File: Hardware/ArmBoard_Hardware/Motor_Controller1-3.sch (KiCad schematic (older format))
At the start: 27 parts, among them Q31 BUK7M6R3-40EX, Q32 BUK7M6R3-40EX, Q33 BUK7M6R3-40EX, U3 VNH5019A_E, U4 VNH5019A_E, U5 VNH5019A_E

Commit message: need to change the mosfet and the other footrpints under it
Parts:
- R40, R41, R42, R43, R44, R45, R46, R47, R48, R49, R50, R51, R52, R53, R54, R55, R56, R57, R58, R59, R60: footprint (none) -> Resistor_SMD:R_0603_1608Metric_Pad0.98x0.95mm_HandSolder
- U3, U4, U5: footprint (none) -> MRDT_ICs:MultiPowerSO_30
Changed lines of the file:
@@
 F 0 "U5" H 3550 4137 60  0000 C CNN
 F 1 "VNH5019A_E" H 3550 4031 60  0000 C CNN
-F 2 "" H 2950 3750 60  0001 C CNN
+F 2 "MRDT_ICs:MultiPowerSO_30" H 2950 3750 60  0001 C CNN
 F 3 "" H 2950 3750 60  0001 C CNN
 	1    2950 2450
@@
 F 0 "R60" H 2700 1350 50  0000 R CNN
 F 1 "3.3k" H 2700 1450 50  0000 R CNN
-F 2 "" H 2500 1400 50  0001 C CNN
+F 2 "Resistor_SMD:R_0603_1608Metric_Pad0.98x0.95mm_HandSolder" H 2500 1400 50  0001 C CNN
 F 3 "~" H 2500 1400 50  0001 C CNN
 	1    2500 1400
@@
 F 0 "R57" V 2450 1550 50  0000 C CNN
 F 1 "1k" V 2350 1550 50  0000 C CNN
-F 2 "" H 2350 1550 50  0001 C CNN
+F 2 "Resistor_SMD:R_0603_1608Metric_Pad0.98x0.95mm_HandSolder" H 2350 1550 50  0001 C CNN
 F 3 "~" H 2350 1550 50  0001 C CNN
 	1    2350 1550
@@
 F 0 "R52" H 2309 2646 50  0000 L CNN
 F 1 "3.3k" H 2309 2555 50  0000 L CNN
-F 2 "" H 2250 2600 50  0001 C CNN
+F 2 "Resistor_SMD:R_0603_1608Metric_Pad0.98x0.95mm_HandSolder" H 2250 2600 50  0001 C CNN
 F 3 "~" H 2250 2600 50  0001 C CNN
 	1    2250 2600
@@
 F 0 "R48" V 2200 2750 50  0000 C CNN
 F 1 "1k" V 2100 2750 50  0000 C CNN
-F 2 "" H 2100 2750 50  0001 C CNN
+F 2 "Resistor_SMD:R_0603_1608Metric_Pad0.98x0.95mm_HandSolder" H 2100 2750 50  0001 C CNN
 F 3 "~" H 2100 2750 50  0001 C CNN
 	1    2100 2750
@@
 F 0 "U3" H 3450 8787 60  0000 C CNN
 F 1 "VNH5019A_E" H 3450 8681 60  0000 C CNN
-F 2 "" H 2850 8400 60  0001 C CNN
+F 2 "MRDT_ICs:MultiPowerSO_30" H 2850 8400 60  0001 C CNN
 F 3 "" H 2850 8400 60  0001 C CNN
 	1    2850 7100
@@
 F 0 "R58" H 2600 6000 50  0000 R CNN
 F 1 "3.3k" H 2600 6100 50  0000 R CNN
-F 2 "" H 2400 6050 50  0001 C CNN
+F 2 "Resistor_SMD:R_0603_1608Metric_Pad0.98x0.95mm_HandSolder" H 2400 6050 50  0001 C CNN
 F 3 "~" H 2400 6050 50  0001 C CNN
 	1    2400 6050
@@
 F 0 "R54" V 2350 6200 50  0000 C CNN
 F 1 "1k" V 2250 6200 50  0000 C CNN
-F 2 "" H 2250 6200 50  0001 C CNN
+F 2 "Resistor_SMD:R_0603_1608Metric_Pad0.98x0.95mm_HandSolder" H 2250 6200 50  0001 C CNN
 F 3 "~" H 2250 6200 50  0001 C CNN
 	1    2250 6200
@@
 F 0 "R49" H 2209 7296 50  0000 L CNN
 F 1 "3.3k" H 2209 7205 50  0000 L CNN
-F 2 "" H 2150 7250 50  0001 C CNN
+F 2 "Resistor_SMD:R_0603_1608Metric_Pad0.98x0.95mm_HandSolder" H 2150 7250 50  0001 C CNN
 F 3 "~" H 2150 7250 50  0001 C CNN
 	1    2150 7250
@@
 F 0 "R44" V 2100 7400 50  0000 C CNN
 F 1 "1k" V 2000 7400 50  0000 C CNN
-F 2 "" H 2000 7400 50  0001 C CNN
+F 2 "Resistor_SMD:R_0603_1608Metric_Pad0.98x0.95mm_HandSolder" H 2000 7400 50  0001 C CNN
 F 3 "~" H 2000 7400 50  0001 C CNN
 	1    2000 7400
@@
 F 0 "U4" H 3500 6437 60  0000 C CNN
 F 1 "VNH5019A_E" H 3500 6331 60  0000 C CNN
-F 2 "" H 2900 6050 60  0001 C CNN
+F 2 "MRDT_ICs:MultiPowerSO_30" H 2900 6050 60  0001 C CNN
 F 3 "" H 2900 6050 60  0001 C CNN
 	1    2900 4750
@@
 F 0 "R59" H 2650 3650 50  0000 R CNN
 F 1 "3.3k" H 2650 3750 50  0000 R CNN
-F 2 "" H 2450 3700 50  0001 C CNN
+F 2 "Resistor_SMD:R_0603_1608Metric_Pad0.98x0.95mm_HandSolder" H 2450 3700 50  0001 C CNN
 F 3 "~" H 2450 3700 50  0001 C CNN
 	1    2450 3700
@@
 F 0 "R56" V 2400 3850 50  0000 C CNN
 F 1 "1k" V 2300 3850 50  0000 C CNN
-F 2 "" H 2300 3850 50  0001 C CNN
+F 2 "Resistor_SMD:R_0603_1608Metric_Pad0.98x0.95mm_HandSolder" H 2300 3850 50  0001 C CNN
 F 3 "~" H 2300 3850 50  0001 C CNN
 	1    2300 3850
@@
 F 0 "R50" H 2259 4946 50  0000 L CNN
 F 1 "3.3k" H 2259 4855 50  0000 L CNN
-F 2 "" H 2200 4900 50  0001 C CNN
+F 2 "Resistor_SMD:R_0603_1608Metric_Pad0.98x0.95mm_HandSolder" H 2200 4900 50  0001 C CNN
 F 3 "~" H 2200 4900 50  0001 C CNN
 	1    2200 4900
@@
 F 0 "R47" V 2150 5050 50  0000 C CNN
 F 1 "1k" V 2050 5050 50  0000 C CNN
-F 2 "" H 2050 5050 50  0001 C CNN
+F 2 "Resistor_SMD:R_0603_1608Metric_Pad0.98x0.95mm_HandSolder" H 2050 5050 50  0001 C CNN
 F 3 "~" H 2050 5050 50  0001 C CNN
 	1    2050 5050
@@
 F 0 "R43" V 1900 4400 50  0000 C CNN
 F 1 "1k" V 2000 4400 50  0000 C CNN
-F 2 "" H 2000 4400 50  0001 C CNN
+F 2 "Resistor_SMD:R_0603_1608Metric_Pad0.98x0.95mm_HandSolder" H 2000 4400 50  0001 C CNN
 F 3 "~" H 2000 4400 50  0001 C CNN
 	1    2000 4400
@@
 F 0 "R42" V 1900 4150 50  0000 C CNN
 F 1 "1k" V 2000 4150 50  0000 C CNN
-F 2 "" H 2000 4150 50  0001 C CNN
+F 2 "Resistor_SMD:R_0603_1608Metric_Pad0.98x0.95mm_HandSolder" H 2000 4150 50  0001 C CNN
 F 3 "~" H 2000 4150 50  0001 C CNN
 	1    2000 4150
@@
 F 0 "R53" V 2150 4300 50  0000 C CNN
 F 1 "1k" V 2250 4300 50  0000 C CNN
-F 2 "" H 2250 4300 50  0001 C CNN
+F 2 "Resistor_SMD:R_0603_1608Metric_Pad0.98x0.95mm_HandSolder" H 2250 4300 50  0001 C CNN
 F 3 "~" H 2250 4300 50  0001 C CNN
 	1    2250 4300
@@
 F 0 "R41" V 1850 6750 50  0000 C CNN
 F 1 "1k" V 1950 6750 50  0000 C CNN
-F 2 "" H 1950 6750 50  0001 C CNN
+F 2 "Resistor_SMD:R_0603_1608Metric_Pad0.98x0.95mm_HandSolder" H 1950 6750 50  0001 C CNN
 F 3 "~" H 1950 6750 50  0001 C CNN
 	1    1950 6750
@@
 F 0 "R40" V 1850 6500 50  0000 C CNN
 F 1 "1k" V 1950 6500 50  0000 C CNN
-F 2 "" H 1950 6500 50  0001 C CNN
+F 2 "Resistor_SMD:R_0603_1608Metric_Pad0.98x0.95mm_HandSolder" H 1950 6500 50  0001 C CNN
 F 3 "~" H 1950 6500 50  0001 C CNN
 	1    1950 6500
@@
 F 0 "R51" V 2100 6650 50  0000 C CNN
 F 1 "1k" V 2200 6650 50  0000 C CNN
-F 2 "" H 2200 6650 50  0001 C CNN
+F 2 "Resistor_SMD:R_0603_1608Metric_Pad0.98x0.95mm_HandSolder" H 2200 6650 50  0001 C CNN
 F 3 "~" H 2200 6650 50  0001 C CNN
 	1    2200 6650
@@
 F 0 "R46" V 1950 2100 50  0000 C CNN
 F 1 "1k" V 2050 2100 50  0000 C CNN
-F 2 "" H 2050 2100 50  0001 C CNN
+F 2 "Resistor_SMD:R_0603_1608Metric_Pad0.98x0.95mm_HandSolder" H 2050 2100 50  0001 C CNN
 F 3 "~" H 2050 2100 50  0001 C CNN
 	1    2050 2100
@@
 F 0 "R45" V 1950 1850 50  0000 C CNN
 F 1 "1k" V 2050 1850 50  0000 C CNN
-F 2 "" H 2050 1850 50  0001 C CNN
+F 2 "Resistor_SMD:R_0603_1608Metric_Pad0.98x0.95mm_HandSolder" H 2050 1850 50  0001 C CNN
 F 3 "~" H 2050 1850 50  0001 C CNN
 	1    2050 1850
@@
 F 0 "R55" V 2200 2000 50  0000 C CNN
 F 1 "1k" V 2300 2000 50  0000 C CNN
-F 2 "" H 2300 2000 50  0001 C CNN
+F 2 "Resistor_SMD:R_0603_1608Metric_Pad0.98x0.95mm_HandSolder" H 2300 2000 50  0001 C CNN
 F 3 "~" H 2300 2000 50  0001 C CNN
 	1    2300 2000

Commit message: late night with the boy
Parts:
- removed Q31, Q32, Q33: BUK7M6R3-40EX, Package_TO_SOT_SMD:LFPAK33, symbol Transistor_FET:BUK7M6R3-40EX
- removed R40, R41, R42, R43, R44, R45, R46, R47, R48, R51, R53, R54, R55, R56, R57: 1k, Resistor_SMD:R_0603_1608Metric_Pad0.98x0.95mm_HandSolder, symbol Device:R_Small
- removed R49, R50, R52, R58, R59, R60: 3.3k, Resistor_SMD:R_0603_1608Metric_Pad0.98x0.95mm_HandSolder, symbol Device:R_Small
- removed U3, U4, U5: VNH5019A_E, MRDT_ICs:MultiPowerSO_30, symbol ArmBoard_Hardware-rescue:VNH5019A_E-MRDT_ICs
- added C5, C6, C7: C_Small, Capacitor_SMD:C_0603_1608Metric_Pad1.08x0.95mm_HandSolder, symbol Device:C_Small
- added R26, R27, R32: 20k, Resistor_SMD:R_0603_1608Metric_Pad0.98x0.95mm_HandSolder, symbol Device:R
- added R28, R29, R30, R31, R33, R34: 1k, Resistor_SMD:R_0603_1608Metric_Pad0.98x0.95mm_HandSolder, symbol Device:R_Small
- added U4, U5, U8: LTC6900, Package_TO_SOT_SMD:SOT-23-5_HandSoldering, symbol MRDT_Devices:LTC6900
- added U6, U7, U9: TB67H400AFNG,EL, MRDT_ICs:TB67H400AFNG,EL, symbol MRDT_ICs:TB67H400AFNG,EL
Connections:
- net labels added: +5V
- net labels removed: +3.3V, ENa_1, ENa_2, ENa_3, ENb_1, ENb_2, ENb_3
- wire segments 228 -> 165
- no-connect marks 0 -> 12

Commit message: Fixed Oscillators
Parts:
- C5, C6, C7: value C_Small -> .1uF
- U4, U5, U8: symbol MRDT_Devices:LTC6900 -> ArmBoard_Hardware-rescue:LTC6900-MRDT_Devices
- U6, U7, U9: symbol MRDT_ICs:TB67H400AFNG,EL -> ArmBoard_Hardware-rescue:TB67H400AFNG,EL-MRDT_ICs
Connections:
- net +5V: now also R26.1, R27.2, R32.2
- net GND: now also C5.2, C6.2, C7.2
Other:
- moved on the sheet: C5, C6, C7, R27
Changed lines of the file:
@@
 	1035 775  1035 740
 Wire Wire Line
-	825  775  1035 775
+	705  775  880  775
 Wire Wire Line
 	1210 775  1210 925
@@
 $EndComp
 Wire Wire Line
-	825  1125 830  1125
-Wire Wire Line
-	825  975  825  1125
+	880  1125 890  1125
 $Comp
 L Device:C_Small C6
 U 1 1 61CA53E2
-P 825 875
-F 0 "C6" H 917 921 50  0000 L CNN
-F 1 "C_Small" H 917 830 50  0000 L CNN
-F 2 "Capacitor_SMD:C_0603_1608Metric_Pad1.08x0.95mm_HandSolder" H 825 875 50  0001 C CNN
-F 3 "~" H 825 875 50  0001 C CNN
-	1    825  875
-	1    0    0    -1
-$EndComp
-Wire Wire Line
-	1130 1125 1210 1125
-$Comp
-L Device:R R27
-U 1 1 61AA62F2
-P 980 1125
-F 0 "R27" V 1187 1125 50  0000 C CNN
-F 1 "20k" V 1096 1125 50  0000 C CNN
-F 2 "Resistor_SMD:R_0603_1608Metric_Pad0.98x0.95mm_HandSolder" V 910 1125 50  0001 C CNN
-F 3 "~" H 980 1125 50  0001 C CNN
-	1    980  1125
-	0    1    1    0
-$EndComp
-Wire Wire Line
-	705  1025 1210 1025
+P 705 875
+F 0 "C6" H 510 935 50  0000 L CNN
+F 1 ".1uF" H 470 875 50  0000 L CNN
+F 2 "Capacitor_SMD:C_0603_1608Metric_Pad1.08x0.95mm_HandSolder" H 705 875 50  0001 C CNN
+F 3 "~" H 705 875 50  0001 C CNN
+	1    705  875
+	1    0    0    -1
+$EndComp
+Wire Wire Line
+	1190 1125 1210 1125
 NoConn ~ 1210 1225
 $Comp
@@
 	1850 1025 2390 1025
 $Comp
-L MRDT_Devices:LTC6900 U5
+L ArmBoard_Hardware-rescue:LTC6900-MRDT_Devices U5
 U 1 1 6198744B
 P 1460 985
+AR Path="/6198744B" Ref="U5"  Part="1"
+AR Path="/63845F20/6198744B" Ref="U5"  Part="1"
 F 0 "U5" H 1530 1270 50  0000 C CNN
 F 1 "LTC6900" H 1530 1179 50  0000 C CNN
@@
 IN_A_2
 $Comp
-L MRDT_ICs:TB67H400AFNG,EL U9
+L ArmBoard_Hardware-rescue:TB67H400AFNG,EL-MRDT_ICs U9
 U 1 1 620C9E6A
 P 8605 2385
@@
 	7580 1435 7805 1435
 $Comp
-L MRDT_Devices:LTC6900 U8
+L ArmBoard_Hardware-rescue:LTC6900-MRDT_Devices U8
 U 1 1 620C9E19
 P 6875 995
+AR Path="/620C9E19" Ref="U8"  Part="1"
+AR Path="/63845F20/620C9E19" Ref="U8"  Part="1"
 F 0 "U8" H 6945 1280 50  0000 C CNN
 F 1 "LTC6900" H 6945 1189 50  0000 C CNN
@@
 L Device:C_Small C7
 U 1 1 620C9DFD
-P 6240 885
-F 0 "C7" H 6332 931 50  0000 L CNN
-F 1 "C_Small" H 6332 840 50  0000 L CNN
-F 2 "Capacitor_SMD:C_0603_1608Metric_Pad1.08x0.95mm_HandSolder" H 6240 885 50  0001 C CNN
-F 3 "~" H 6240 885 50  0001 C CNN
-	1    6240 885
-	1    0    0    -1
-$EndComp
-Wire Wire Line
-	6240 985  6240 1135
+P 6120 895
+F 0 "C7" H 6212 941 50  0000 L CNN
+F 1 ".1uF" H 6212 850 50  0000 L CNN
+F 2 "Capacitor_SMD:C_0603_1608Metric_Pad1.08x0.95mm_HandSolder" H 6120 895 50  0001 C CNN
+F 3 "~" H 6120 895 50  0001 C CNN
+	1    6120 895
+	1    0    0    -1
+$EndComp
 Wire Wire Line
 	6240 1135 6245 1135
@@
 	6625 785  6625 935
 Wire Wire Line
-	6240 785  6450 785
-Wire Wire Line
 	6450 785  6450 750
 Connection ~ 6450 785
@@
 Wire Wire Line
 	815  4725 820  4725
-Wire Wire Line
-	815  4575 815  4725
 $Comp
 L Device:C_Small C5
 U 1 1 621A2B7A
-P 815 4475
-F 0 "C5" H 907 4521 50  0000 L CNN
-F 1 "C_Small" H 907 4430 50  0000 L CNN
-F 2 "Capacitor_SMD:C_0603_1608Metric_Pad1.08x0.95mm_HandSolder" H 815 4475 50  0001 C CNN
-F 3 "~" H 815 4475 50  0001 C CNN
-	1    815  4475
+P 695 4480
+F 0 "C5" H 787 4526 50  0000 L CNN
+F 1 ".1uF" H 787 4435 50  0000 L CNN
+F 2 "Capacitor_SMD:C_0603_1608Metric_Pad1.08x0.95mm_HandSolder" H 695 4480 50  0001 C CNN
+F 3 "~" H 695 4480 50  0001 C CNN
+	1    695  4480
 	1    0    0    -1
 $EndComp
@@
 	1840 4625 2380 4625
 $Comp
-L MRDT_Devices:LTC6900 U4
+L ArmBoard_Hardware-rescue:LTC6900-MRDT_Devices U4
 U 1 1 621A2B96
 P 1450 4585
+AR Path="/621A2B96" Ref="U4"  Part="1"
+AR Path="/63845F20/621A2B96" Ref="U4"  Part="1"
 F 0 "U4" H 1520 4870 50  0000 C CNN
 F 1 "LTC6900" H 1520 4779 50  0000 C CNN
@@
 	3180 7525 3180 7400
 $Comp
-L MRDT_ICs:TB67H400AFNG,EL U6
+L ArmBoard_Hardware-rescue:TB67H400AFNG,EL-MRDT_ICs U6
 U 1 1 621A2BE7
 P 3180 5975
@@
 OUTa_3
 $Comp
-L MRDT_ICs:TB67H400AFNG,EL U7
+L ArmBoard_Hardware-rescue:TB67H400AFNG,EL-MRDT_ICs U7
 U 1 1 61982ADA
 P 3190 2375
@@
 	1    0    0    -1
 $EndComp
+$Comp
+L Device:R R27
+U 1 1 61AA62F2
+P 1040 1125
+F 0 "R27" V 1247 1125 50  0000 C CNN
+F 1 "20k" V 1156 1125 50  0000 C CNN
+F 2 "Resistor_SMD:R_0603_1608Metric_Pad0.98x0.95mm_HandSolder" V 970 1125 50  0001 C CNN
+F 3 "~" H 1040 1125 50  0001 C CNN
+	1    1040 1125
+	0    1    1    0
+$EndComp
+Wire Wire Line
+	705  1025 1210 1025
+Wire Wire Line
+	705  975  705  1025
+Connection ~ 705  1025
+Wire Wire Line
+	880  1125 880  775
+Connection ~ 880  775
+Wire Wire Line
+	880  775  1035 775
+Wire Wire Line
+	695  4580 695  4625
+Connection ~ 695  4625
+Wire Wire Line
+	815  4375 815  4725
+Wire Wire Line
+	815  4375 695  4375
+Wire Wire Line
+	695  4375 695  4380
+Connection ~ 815  4375
+Wire Wire Line
+	6120 795  6120 785
+Wire Wire Line
+	6120 785  6240 785
+Connection ~ 6240 785
+Wire Wire Line
+	6240 785  6450 785
+Wire Wire Line
+	6240 785  6240 1135
+Wire Wire Line
+	6120 995  6120 1035
+Connection ~ 6120 1035
 $EndSCHEMATC

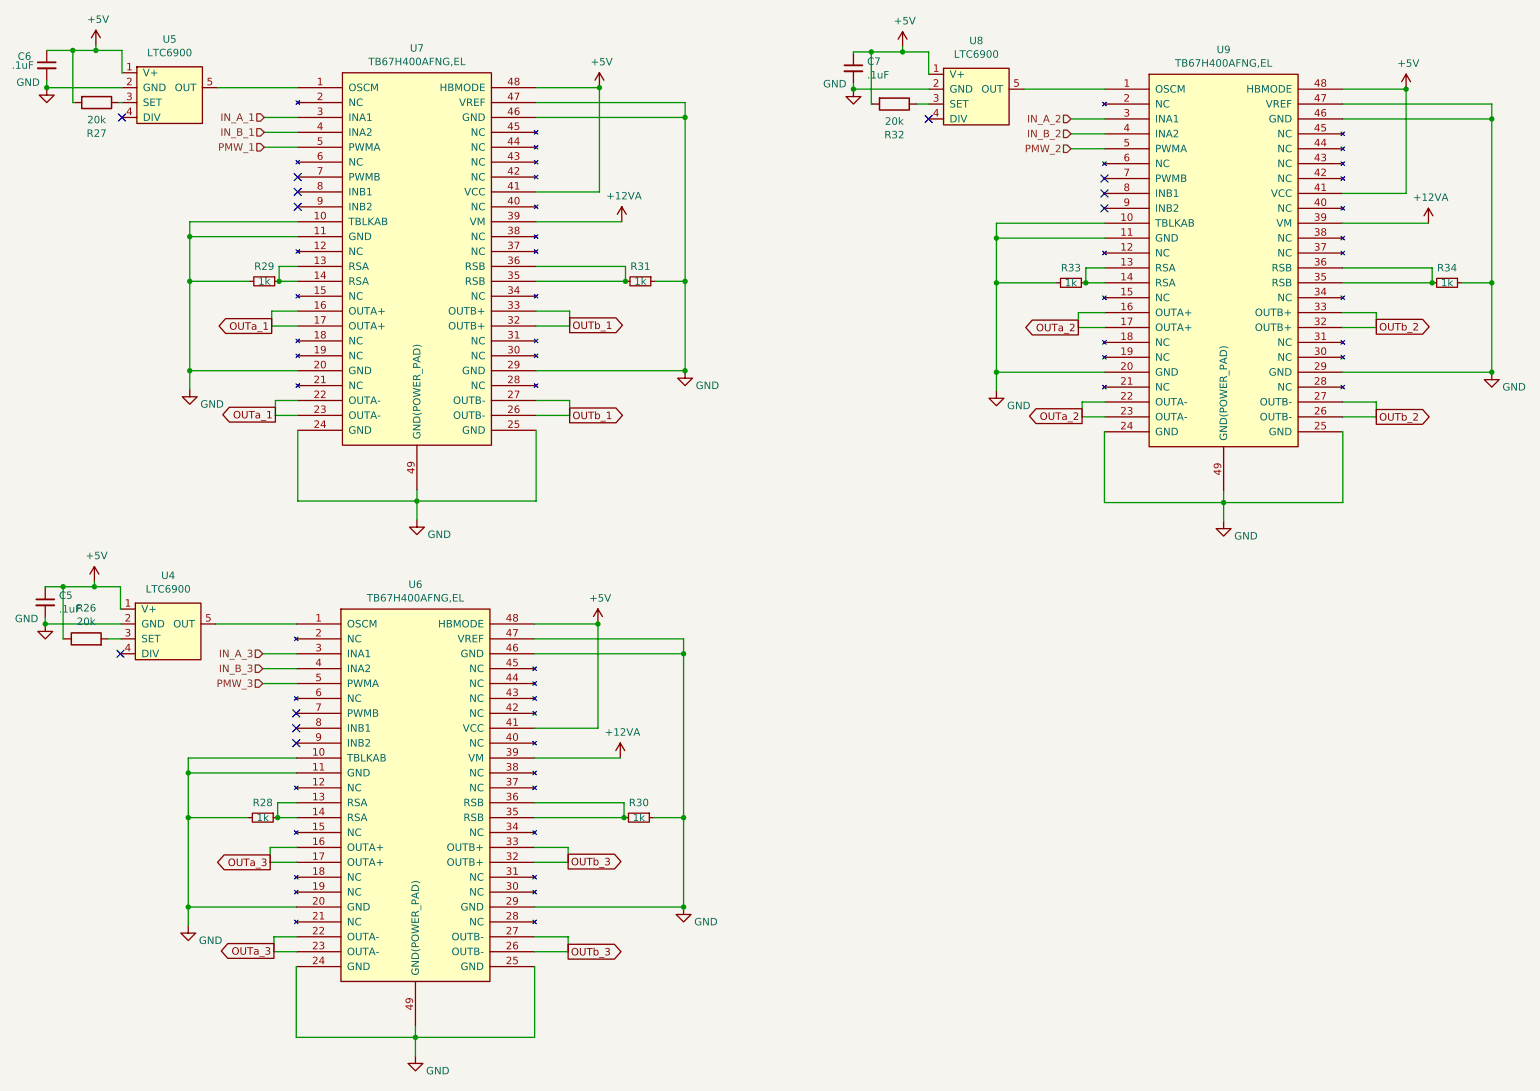
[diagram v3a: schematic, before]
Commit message: armboard review
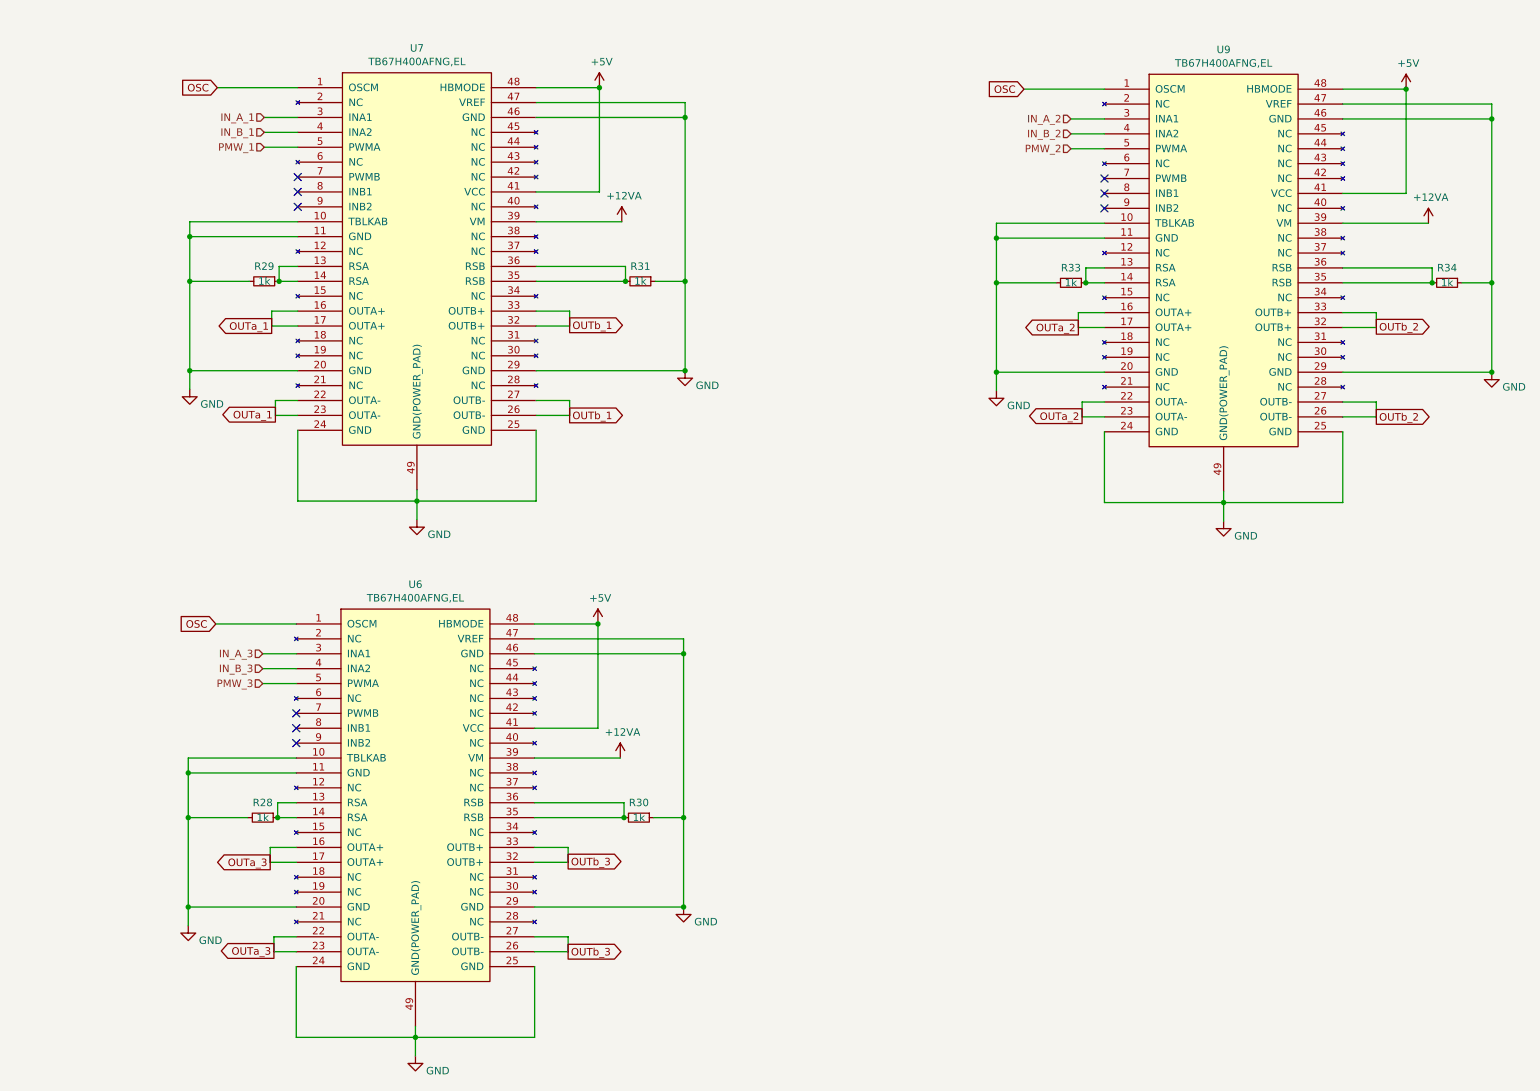
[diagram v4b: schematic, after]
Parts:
- removed C5, C6, C7: .1uF, Capacitor_SMD:C_0603_1608Metric_Pad1.08x0.95mm_HandSolder, symbol Device:C_Small
- removed R26, R27, R32: 20k, Resistor_SMD:R_0603_1608Metric_Pad0.98x0.95mm_HandSolder, symbol Device:R
- removed U4, U5, U8: LTC6900, Package_TO_SOT_SMD:SOT-23-5_HandSoldering, symbol ArmBoard_Hardware-rescue:LTC6900-MRDT_Devices
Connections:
- net OSC: now reaches U7.1 (OSCM)
- net OSC: now also U6.1 (OSCM), U9.1 (OSCM)
- no-connect marks 12 -> 9

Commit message: Rescued the Libaries
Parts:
- U6, U7, U9: symbol ArmBoard_Hardware-rescue:TB67H400AFNG,EL-MRDT_ICs -> MRDT_ICs:TB67H400AFNG,EL
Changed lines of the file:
@@
 IN_A_2
 $Comp
-L ArmBoard_Hardware-rescue:TB67H400AFNG,EL-MRDT_ICs U9
+L MRDT_ICs:TB67H400AFNG,EL U9
 U 1 1 620C9E6A
 P 8605 2385
+AR Path="/620C9E6A" Ref="U9"  Part="1"
+AR Path="/63845F20/620C9E6A" Ref="U9"  Part="1"
 F 0 "U9" H 8605 4000 50  0000 C CNN
 F 1 "TB67H400AFNG,EL" H 8605 3909 50  0000 C CNN
@@
 	3180 7525 3180 7400
 $Comp
-L ArmBoard_Hardware-rescue:TB67H400AFNG,EL-MRDT_ICs U6
+L MRDT_ICs:TB67H400AFNG,EL U6
 U 1 1 621A2BE7
 P 3180 5975
+AR Path="/621A2BE7" Ref="U6"  Part="1"
+AR Path="/63845F20/621A2BE7" Ref="U6"  Part="1"
 F 0 "U6" H 3180 7590 50  0000 C CNN
 F 1 "TB67H400AFNG,EL" H 3180 7499 50  0000 C CNN
@@
 OUTa_3
 $Comp
-L ArmBoard_Hardware-rescue:TB67H400AFNG,EL-MRDT_ICs U7
+L MRDT_ICs:TB67H400AFNG,EL U7
 U 1 1 61982ADA
 P 3190 2375
+AR Path="/61982ADA" Ref="U7"  Part="1"
+AR Path="/63845F20/61982ADA" Ref="U7"  Part="1"
 F 0 "U7" H 3190 3990 50  0000 C CNN
 F 1 "TB67H400AFNG,EL" H 3190 3899 50  0000 C CNN
